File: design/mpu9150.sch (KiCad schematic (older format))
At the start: 8 parts, among them U10 MPU9150

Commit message: initial commit
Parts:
- U10: footprint Housings_DFN_QFN:QFN-24-1EP_3x3mm_Pitch0.4mm -> Housings_DFN_QFN:QFN-24-1EP_4x4mm_Pitch0.5mm
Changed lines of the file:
@@
 F 0 "U10" H 4400 4600 50  0000 L BNN
 F 1 "MPU9150" H 4275 2750 50  0000 L BNN
-F 2 "Housings_DFN_QFN:QFN-24-1EP_3x3mm_Pitch0.4mm" H 3450 4700 50  0001 L BNN
+F 2 "Housings_DFN_QFN:QFN-24-1EP_4x4mm_Pitch0.5mm" H 3450 4700 50  0001 L BNN
 F 3 "" H 3450 4700 50  0001 L BNN
 	1    4475 3775

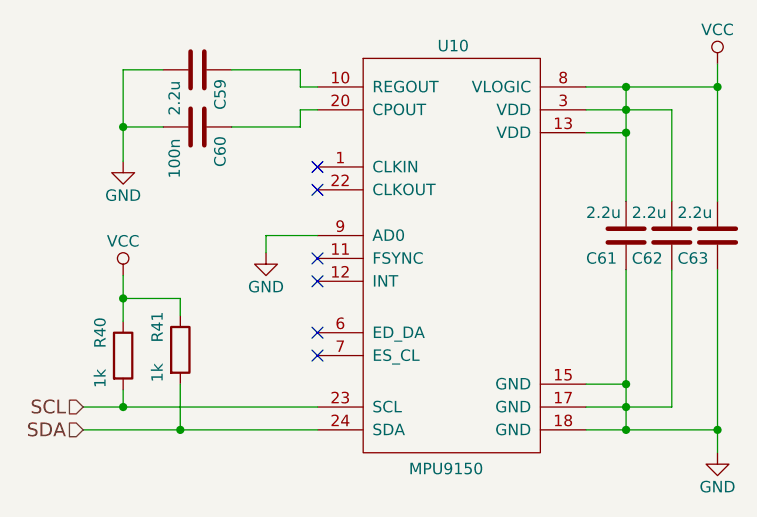
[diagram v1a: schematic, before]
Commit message: initial commit
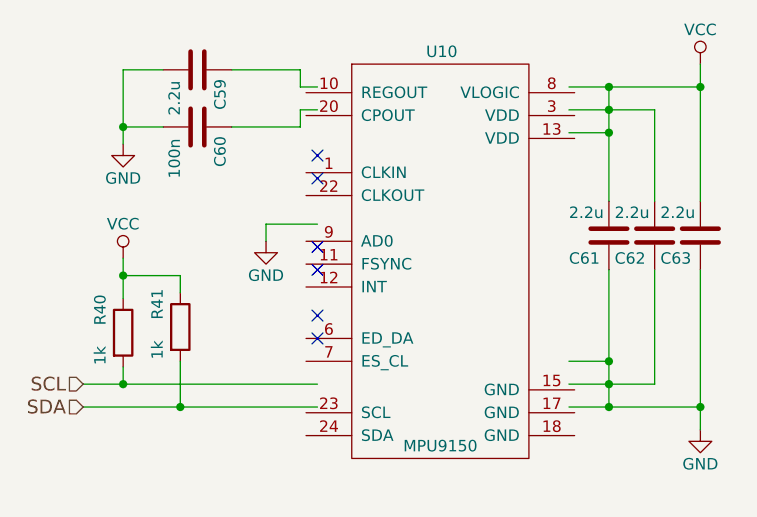
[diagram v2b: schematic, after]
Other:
- moved on the sheet: C61, C62, C63, R40, R41, U10
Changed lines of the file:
@@
 LIBS:valves
 LIBS:crf_1
+LIBS:crf_2
 LIBS:VESC_6-cache
 EELAYER 25 0
@@
 L MPU9150 U10
 U 1 1 5A8CD83F
-P 4475 3775
-F 0 "U10" H 4400 4600 50  0000 L BNN
-F 1 "MPU9150" H 4275 2750 50  0000 L BNN
-F 2 "Housings_DFN_QFN:QFN-24-1EP_4x4mm_Pitch0.5mm" H 3450 4700 50  0001 L BNN
-F 3 "" H 3450 4700 50  0001 L BNN
-	1    4475 3775
-	1    0    0    -1
-$EndComp
-NoConn ~ 3875 4175
-NoConn ~ 3875 4275
-NoConn ~ 3875 3850
-NoConn ~ 3875 3950
-NoConn ~ 3875 3450
-NoConn ~ 3875 3550
+P 4425 3800
+F 0 "U10" H 4350 4625 50  0000 L BNN
+F 1 "MPU9150" H 4250 2900 50  0000 L BNN
+F 2 "Housings_DFN_QFN:QFN-24-1EP_4x4mm_Pitch0.5mm" H 3400 4725 50  0001 L BNN
+F 3 "" H 3400 4725 50  0001 L BNN
+	1    4425 3800
+	1    0    0    -1
+$EndComp
+NoConn ~ 3875 4100
+NoConn ~ 3875 4200
+NoConn ~ 3875 3800
+NoConn ~ 3875 3900
+NoConn ~ 3875 3400
+NoConn ~ 3875 3500
 $Comp
 L GND #PWR093
 U 1 1 5A8CDBDA
-P 3650 3825
-F 0 "#PWR093" H 3650 3575 50  0001 C CNN
-F 1 "GND" H 3650 3675 50  0000 C CNN
-F 2 "" H 3650 3825 50  0001 C CNN
-F 3 "" H 3650 3825 50  0001 C CNN
-	1    3650 3825
+P 3650 3775
+F 0 "#PWR093" H 3650 3525 50  0001 C CNN
+F 1 "GND" H 3650 3625 50  0000 C CNN
+F 2 "" H 3650 3775 50  0001 C CNN
+F 3 "" H 3650 3775 50  0001 C CNN
+	1    3650 3775
 	1    0    0    -1
 $EndComp
@@
 L VCC #PWR094
 U 1 1 5A8CDC21
-P 3025 3925
-F 0 "#PWR094" H 3025 3775 50  0001 C CNN
-F 1 "VCC" H 3025 4075 50  0000 C CNN
-F 2 "" H 3025 3925 50  0001 C CNN
-F 3 "" H 3025 3925 50  0001 C CNN
-	1    3025 3925
+P 3025 3850
+F 0 "#PWR094" H 3025 3700 50  0001 C CNN
+F 1 "VCC" H 3025 4000 50  0000 C CNN
+F 2 "" H 3025 3850 50  0001 C CNN
+F 3 "" H 3025 3850 50  0001 C CNN
+	1    3025 3850
 	1    0    0    -1
 $EndComp
@@
 L R R40
 U 1 1 5A8CDC61
-P 3025 4275
-F 0 "R40" V 2925 4375 50  0000 C CNN
-F 1 "1k" V 2925 4175 50  0000 C CNN
-F 2 "CRF1:SMD-0603_r" V 2955 4275 50  0001 C CNN
-F 3 "" H 3025 4275 50  0001 C CNN
-	1    3025 4275
-	1    0    0    -1
-$EndComp
+P 3025 4175
+F 0 "R40" V 2925 4275 50  0000 C CNN
+F 1 "1k" V 2925 4075 50  0000 C CNN
+F 2 "CRF1:SMD-0603_r" V 2955 4175 50  0001 C CNN
+F 3 "" H 3025 4175 50  0001 C CNN
+	1    3025 4175
+	1    0    0    -1
+$EndComp
+Text HLabel 2850 4400 0    60   Input ~ 0
+SCL
 Text HLabel 2850 4500 0    60   Input ~ 0
-SCL
-Text HLabel 2850 4600 0    60   Input ~ 0
 SDA
-Wire Wire Line
-	3875 3750 3650 3750
-Wire Wire Line
-	3650 3750 3650 3825
-Wire Wire Line
-	2850 4600 3875 4600
-Wire Wire Line
-	3275 4600 3275 4400
-Wire Wire Line
-	3025 3925 3025 4125
-Wire Wire Line
-	3025 4025 3275 4025
-Wire Wire Line
-	3275 4025 3275 4100
-Wire Wire Line
-	2850 4500 3875 4500
-Wire Wire Line
-	3025 4500 3025 4425
-Connection ~ 3025 4025
-Connection ~ 3025 4500
-Connection ~ 3275 4600
 $Comp
 L R R41
 U 1 1 5A8CDFDA
-P 3275 4250
-F 0 "R41" V 3175 4350 50  0000 C CNN
-F 1 "1k" V 3175 4150 50  0000 C CNN
-F 2 "CRF1:SMD-0603_r" V 3205 4250 50  0001 C CNN
-F 3 "" H 3275 4250 50  0001 C CNN
-	1    3275 4250
+P 3275 4150
+F 0 "R41" V 3175 4250 50  0000 C CNN
+F 1 "1k" V 3175 4050 50  0000 C CNN
+F 2 "CRF1:SMD-0603_r" V 3205 4150 50  0001 C CNN
+F 3 "" H 3275 4150 50  0001 C CNN
+	1    3275 4150
 	1    0    0    -1
 $EndComp
@@
 L C C61
 U 1 1 5A8CE39F
-P 5225 3750
-F 0 "C61" H 5050 3650 50  0000 L CNN
-F 1 "2.2u" H 5050 3850 50  0000 L CNN
-F 2 "CRF1:SMD-0603_c" H 5263 3600 50  0001 C CNN
-F 3 "" H 5225 3750 50  0001 C CNN
-	1    5225 3750
+P 5150 3750
+F 0 "C61" H 4975 3650 50  0000 L CNN
+F 1 "2.2u" H 4975 3850 50  0000 L CNN
+F 2 "CRF1:SMD-0603_c" H 5188 3600 50  0001 C CNN
+F 3 "" H 5150 3750 50  0001 C CNN
+	1    5150 3750
 	1    0    0    -1
 $EndComp
@@
 L C C62
 U 1 1 5A8CE4DF
-P 5425 3750
-F 0 "C62" H 5250 3650 50  0000 L CNN
-F 1 "2.2u" H 5250 3850 50  0000 L CNN
-F 2 "CRF1:SMD-0603_c" H 5463 3600 50  0001 C CNN
-F 3 "" H 5425 3750 50  0001 C CNN
-	1    5425 3750
+P 5350 3750
+F 0 "C62" H 5175 3650 50  0000 L CNN
+F 1 "2.2u" H 5175 3850 50  0000 L CNN
+F 2 "CRF1:SMD-0603_c" H 5388 3600 50  0001 C CNN
+F 3 "" H 5350 3750 50  0001 C CNN
+	1    5350 3750
 	1    0    0    -1
 $EndComp
@@
 L C C63
 U 1 1 5A8CE506
-P 5625 3750
-F 0 "C63" H 5450 3650 50  0000 L CNN
-F 1 "2.2u" H 5450 3850 50  0000 L CNN
-F 2 "CRF1:SMD-0603_c" H 5663 3600 50  0001 C CNN
-F 3 "" H 5625 3750 50  0001 C CNN
-	1    5625 3750
-	1    0    0    -1
-$EndComp
-Wire Wire Line
-	5050 3100 5625 3100
-Wire Wire Line
-	5225 3100 5225 3600
-Wire Wire Line
-	5225 3900 5225 4600
-Wire Wire Line
-	5050 4600 5625 4600
-Wire Wire Line
-	5050 4500 5425 4500
-Connection ~ 5225 4500
-Wire Wire Line
-	5050 4400 5225 4400
-Connection ~ 5225 4400
-Wire Wire Line
-	5050 3200 5425 3200
-Connection ~ 5225 3200
-Wire Wire Line
-	5050 3300 5225 3300
-Connection ~ 5225 3300
-Wire Wire Line
-	5425 3200 5425 3600
-Wire Wire Line
-	5425 4500 5425 3900
-Wire Wire Line
-	5625 3900 5625 4700
-Connection ~ 5225 4600
-Wire Wire Line
-	5625 3000 5625 3600
-Connection ~ 5225 3100
+P 5550 3750
+F 0 "C63" H 5375 3650 50  0000 L CNN
+F 1 "2.2u" H 5375 3850 50  0000 L CNN
+F 2 "CRF1:SMD-0603_c" H 5588 3600 50  0001 C CNN
+F 3 "" H 5550 3750 50  0001 C CNN
+	1    5550 3750
+	1    0    0    -1
+$EndComp
 $Comp
 L VCC #PWR095
 U 1 1 5A8CE66F
-P 5625 3000
-F 0 "#PWR095" H 5625 2850 50  0001 C CNN
-F 1 "VCC" H 5625 3150 50  0000 C CNN
-F 2 "" H 5625 3000 50  0001 C CNN
-F 3 "" H 5625 3000 50  0001 C CNN
-	1    5625 3000
-	1    0    0    -1
-$EndComp
-Connection ~ 5625 3100
+P 5550 3000
+F 0 "#PWR095" H 5550 2850 50  0001 C CNN
+F 1 "VCC" H 5550 3150 50  0000 C CNN
+F 2 "" H 5550 3000 50  0001 C CNN
+F 3 "" H 5550 3000 50  0001 C CNN
+	1    5550 3000
+	1    0    0    -1
+$EndComp
 $Comp
 L GND #PWR096
 U 1 1 5A8CE6B3
-P 5625 4700
-F 0 "#PWR096" H 5625 4450 50  0001 C CNN
-F 1 "GND" H 5625 4550 50  0000 C CNN
-F 2 "" H 5625 4700 50  0001 C CNN
-F 3 "" H 5625 4700 50  0001 C CNN
-	1    5625 4700
-	1    0    0    -1
-$EndComp
-Connection ~ 5625 4600
+P 5550 4600
+F 0 "#PWR096" H 5550 4350 50  0001 C CNN
+F 1 "GND" H 5550 4450 50  0000 C CNN
+F 2 "" H 5550 4600 50  0001 C CNN
+F 3 "" H 5550 4600 50  0001 C CNN
+	1    5550 4600
+	1    0    0    -1
+$EndComp
 $Comp
 L C C59
@@
 	0    -1   -1   0
 $EndComp
-Wire Wire Line
-	3875 3100 3800 3100
-Wire Wire Line
-	3800 3100 3800 3025
-Wire Wire Line
-	3800 3025 3500 3025
 $Comp
 L C C60
@@
 	0    -1   -1   0
 $EndComp
-Wire Wire Line
-	3875 3200 3800 3200
-Wire Wire Line
-	3800 3200 3800 3275
-Wire Wire Line
-	3800 3275 3500 3275
 $Comp
 L GND #PWR097
 U 1 1 5A8CE8A1
-P 3025 3425
-F 0 "#PWR097" H 3025 3175 50  0001 C CNN
-F 1 "GND" H 3025 3275 50  0000 C CNN
-F 2 "" H 3025 3425 50  0001 C CNN
-F 3 "" H 3025 3425 50  0001 C CNN
-	1    3025 3425
-	1    0    0    -1
-$EndComp
+P 3025 3350
+F 0 "#PWR097" H 3025 3100 50  0001 C CNN
+F 1 "GND" H 3025 3200 50  0000 C CNN
+F 2 "" H 3025 3350 50  0001 C CNN
+F 3 "" H 3025 3350 50  0001 C CNN
+	1    3025 3350
+	1    0    0    -1
+$EndComp
+Wire Wire Line
+	3875 3700 3650 3700
+Wire Wire Line
+	3650 3700 3650 3775
+Wire Wire Line
+	2850 4500 3875 4500
+Wire Wire Line
+	3275 4500 3275 4300
+Wire Wire Line
+	3025 3850 3025 4025
+Wire Wire Line
+	3025 3925 3275 3925
+Wire Wire Line
+	3275 3925 3275 4000
+Wire Wire Line
+	2850 4400 3875 4400
+Wire Wire Line
+	3025 4400 3025 4325
+Connection ~ 3025 3925
+Connection ~ 3025 4400
+Connection ~ 3275 4500
+Wire Wire Line
+	4975 3100 5550 3100
+Wire Wire Line
+	5150 3100 5150 3600
+Connection ~ 5150 4500
+Connection ~ 5150 4400
+Wire Wire Line
+	4975 3200 5350 3200
+Connection ~ 5150 3200
+Wire Wire Line
+	4975 3300 5150 3300
+Connection ~ 5150 3300
+Wire Wire Line
+	5350 3200 5350 3600
+Wire Wire Line
+	5550 3000 5550 3600
+Connection ~ 5150 3100
+Connection ~ 5550 3100
+Wire Wire Line
+	3875 3100 3800 3100
+Wire Wire Line
+	3800 3100 3800 3025
+Wire Wire Line
+	3800 3025 3500 3025
+Wire Wire Line
+	3875 3200 3800 3200
+Wire Wire Line
+	3800 3200 3800 3275
+Wire Wire Line
+	3800 3275 3500 3275
 Wire Wire Line
 	3200 3025 3025 3025
 Wire Wire Line
-	3025 3025 3025 3425
-Wire Wire Line
-	3200 3275 3025 3275
+	3025 3025 3025 3350
+Wire Wire Line
+	3025 3275 3200 3275
 Connection ~ 3025 3275
+Wire Wire Line
+	4975 4300 5150 4300
+Connection ~ 5150 4300
+Wire Wire Line
+	5150 3900 5150 4500
+Wire Wire Line
+	5350 4400 5350 3900
+Wire Wire Line
+	4975 4400 5350 4400
+Wire Wire Line
+	4975 4500 5550 4500
+Wire Wire Line
+	5550 3900 5550 4600
+Connection ~ 5550 4500
 $EndSCHEMATC

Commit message: initial commit
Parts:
- U10: footprint Housings_DFN_QFN:QFN-24-1EP_4x4mm_Pitch0.5mm -> Housings_DFN_QFN:QFN-24_4x4mm_Pitch0.5mm
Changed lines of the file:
@@
 LIBS:valves
 LIBS:crf_1
-LIBS:crf_2
 LIBS:VESC_6-cache
 EELAYER 25 0
@@
 F 0 "U10" H 4350 4625 50  0000 L BNN
 F 1 "MPU9150" H 4250 2900 50  0000 L BNN
-F 2 "Housings_DFN_QFN:QFN-24-1EP_4x4mm_Pitch0.5mm" H 3400 4725 50  0001 L BNN
+F 2 "Housings_DFN_QFN:QFN-24_4x4mm_Pitch0.5mm" H 3400 4725 50  0001 L BNN
 F 3 "" H 3400 4725 50  0001 L BNN
 	1    4425 3800
